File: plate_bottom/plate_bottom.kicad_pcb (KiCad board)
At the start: 2 copper layers, 173.5 x 138.9 mm, 14 parts

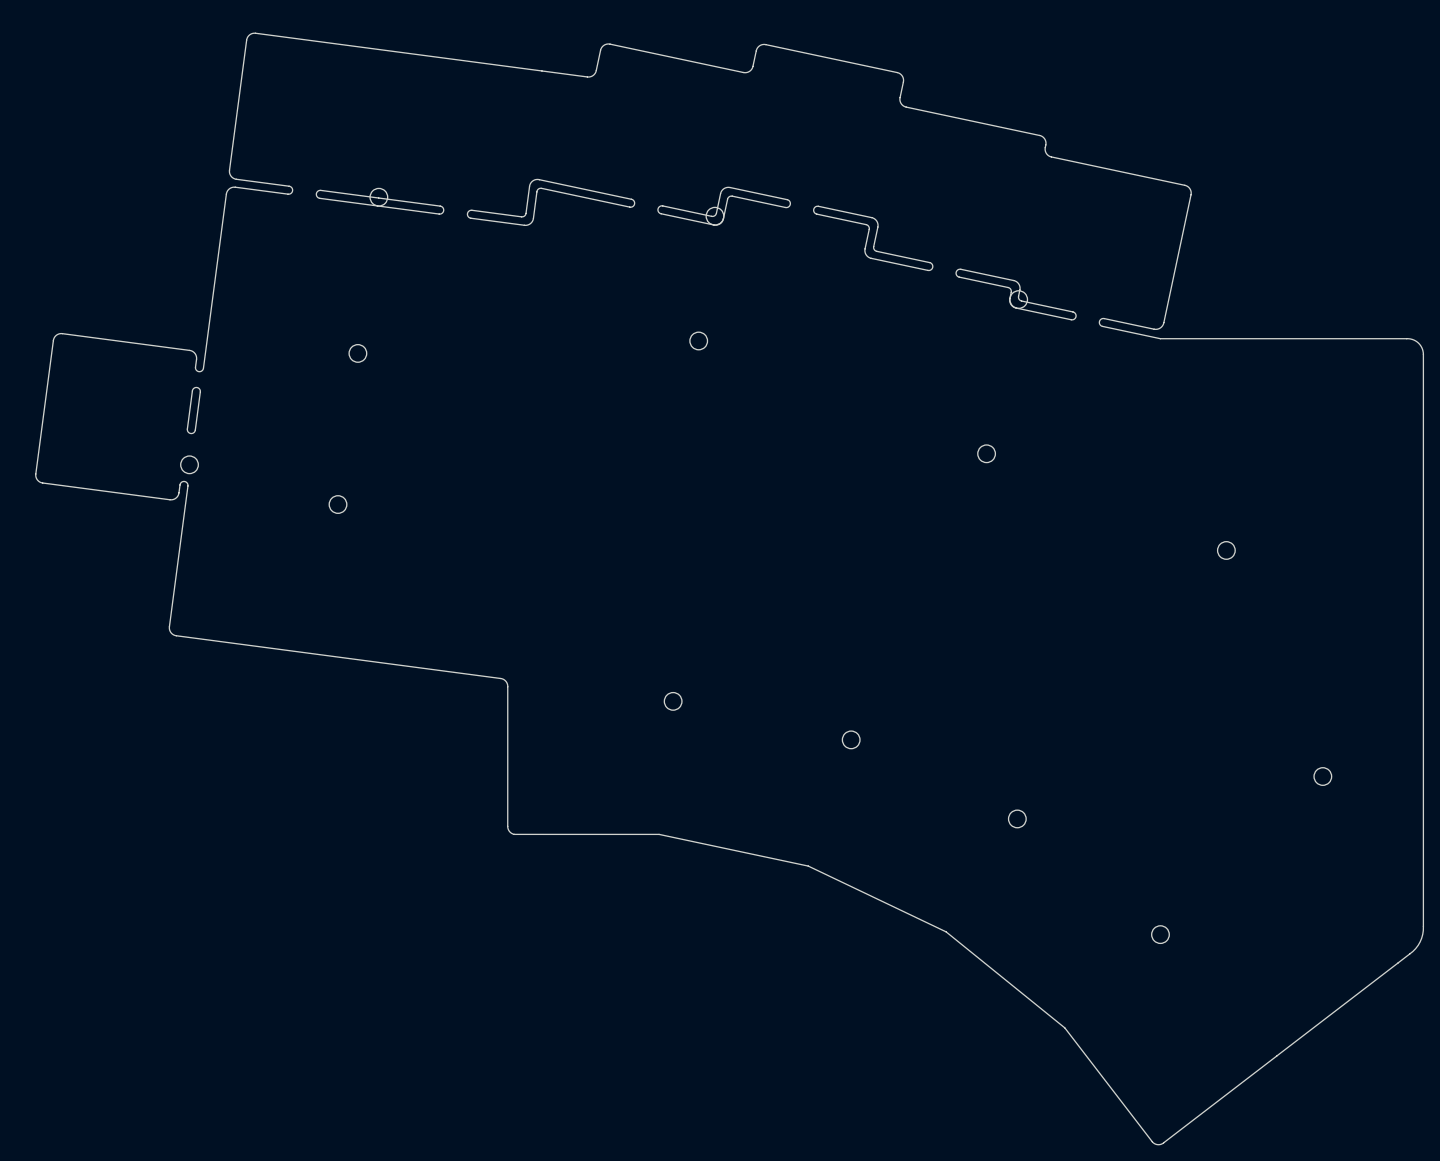
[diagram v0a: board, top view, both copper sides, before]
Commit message: Multiple fixes
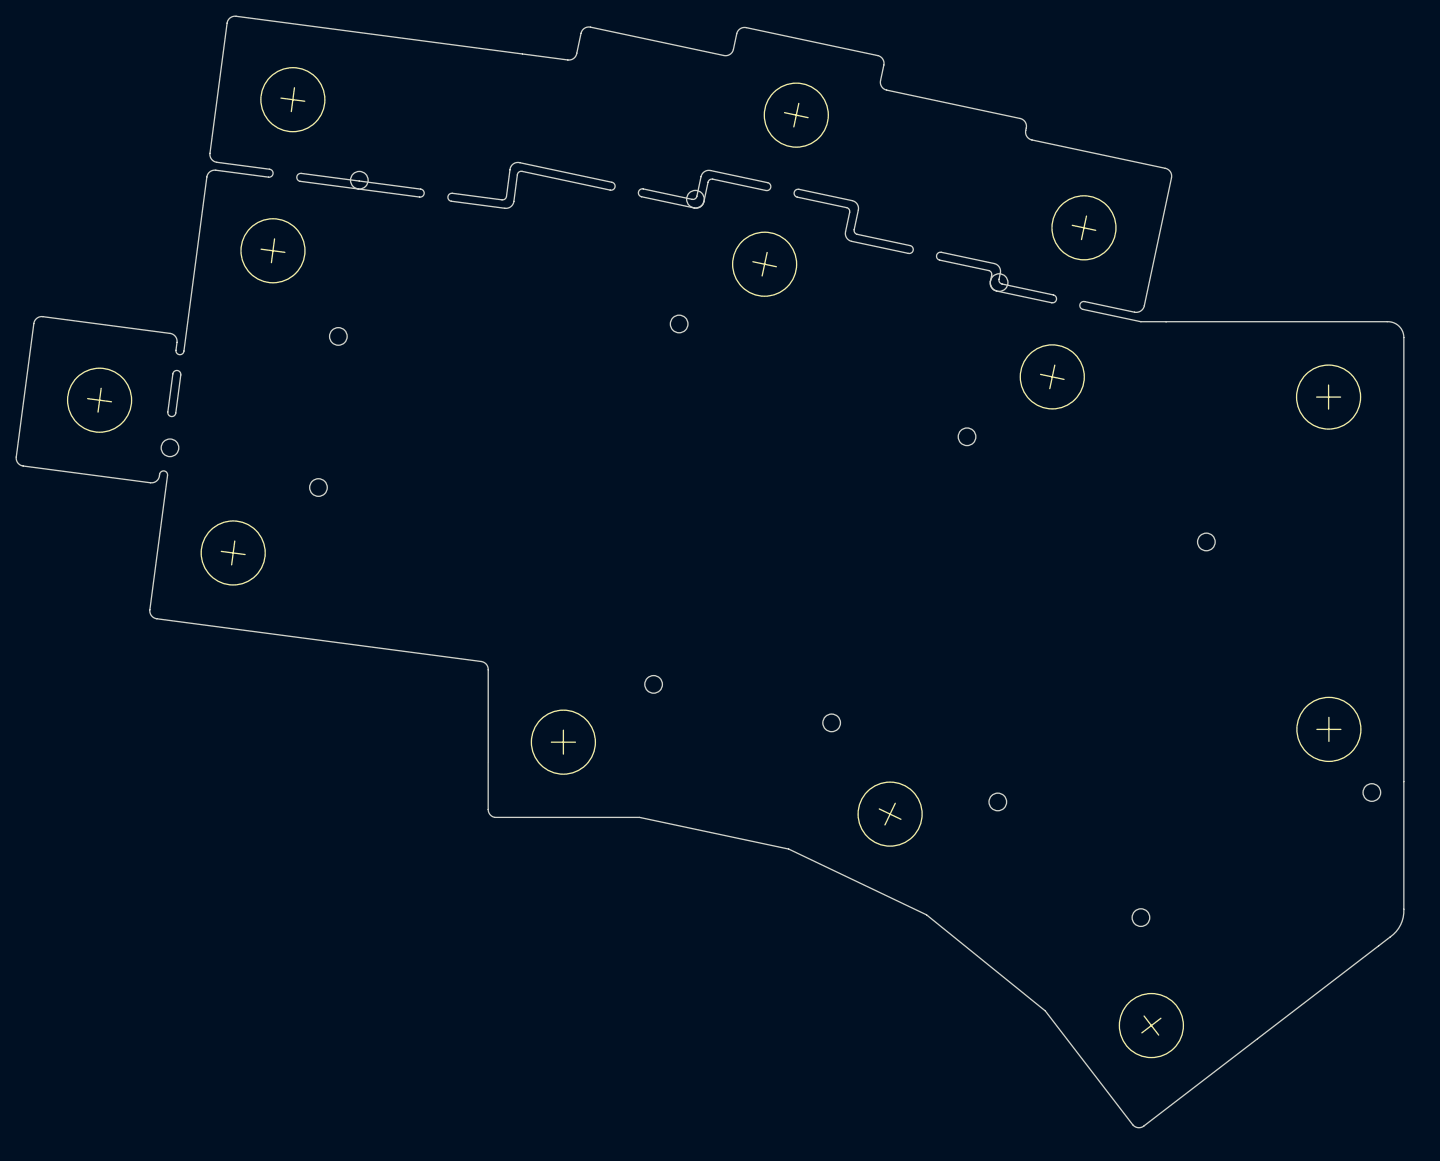
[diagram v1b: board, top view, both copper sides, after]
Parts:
- added SW1: SW_Push, used_footprints:bumpon_mark, F.Cu at (87.9, 30.6)
- added SW10: SW_Push, used_footprints:bumpon_mark, F.Cu at (146.8, 51.2)
- added SW12: SW_Push, used_footprints:bumpon_mark, F.Cu at (217.3, 67.8)
- added SW12: SW_Push, used_footprints:bumpon_mark, F.Cu at (182.8, 65.3)
- added SW19: SW_Push, used_footprints:bumpon_mark, F.Cu at (217.4, 109.3)
- added SW20: SW_Push, used_footprints:bumpon_mark, F.Cu at (80.4, 87.3)
- added SW27: SW_Push, used_footprints:bumpon_mark, F.Cu at (63.7, 68.2)
- added SW28: SW_Push, used_footprints:bumpon_mark, F.Cu at (121.7, 110.9)
- added SW30: SW_Push, used_footprints:bumpon_mark, F.Cu at (162.5, 119.9)
- added SW32: SW_Push, used_footprints:bumpon_mark, F.Cu at (195.2, 146.3)
- added SW4: SW_Push, used_footprints:bumpon_mark, F.Cu at (150.8, 32.5)
- added SW6: SW_Push, used_footprints:bumpon_mark, F.Cu at (186.8, 46.6)
- added SW7: SW_Push, used_footprints:bumpon_mark, F.Cu at (85.4, 49.5)
- moved HM1 6.44 mm to (222.7, 117.2)
- moved HM10 3.24 mm to (172.1, 72.7)
- moved HM11 3.24 mm to (136.2, 58.6)
- moved HM6 3.24 mm to (91.1, 79.1)
- moved HM4 3.24 mm to (155.2, 108.5)
- moved HM7 3.24 mm to (96.2, 40.7)
- moved HM13 3.24 mm to (133.0, 103.7)
- moved HM2 3.24 mm to (176.2, 53.5)
- moved HM9 3.24 mm to (138.2, 43.0)
- moved HM3 3.24 mm to (193.9, 132.8)
- moved HM8 3.24 mm to (93.6, 60.2)
- moved HM14 3.24 mm to (176.0, 118.4)
- moved HM5 3.24 mm to (72.5, 74.1)
- moved H16 2.72 mm to (202.1, 85.9)
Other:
- outline, holes or cut-outs redrawn
